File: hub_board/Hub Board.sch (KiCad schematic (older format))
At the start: 23 parts, among them J1 Conn_01x04, J2 Conn_01x04, J3 Conn_01x04, J4 Conn_01x04, P4 SERIAL, SW1 Switch_SPDT_x2, SW2 Switch_DPST, U0 10118194, U1 LM3671, U3 ESP-12E, U4 DIY-OLED-0.96, U5 SF303GJ26, U6 SN74LVC1T45 - MOSI, U7 SN74LVC1T45 - SCLK

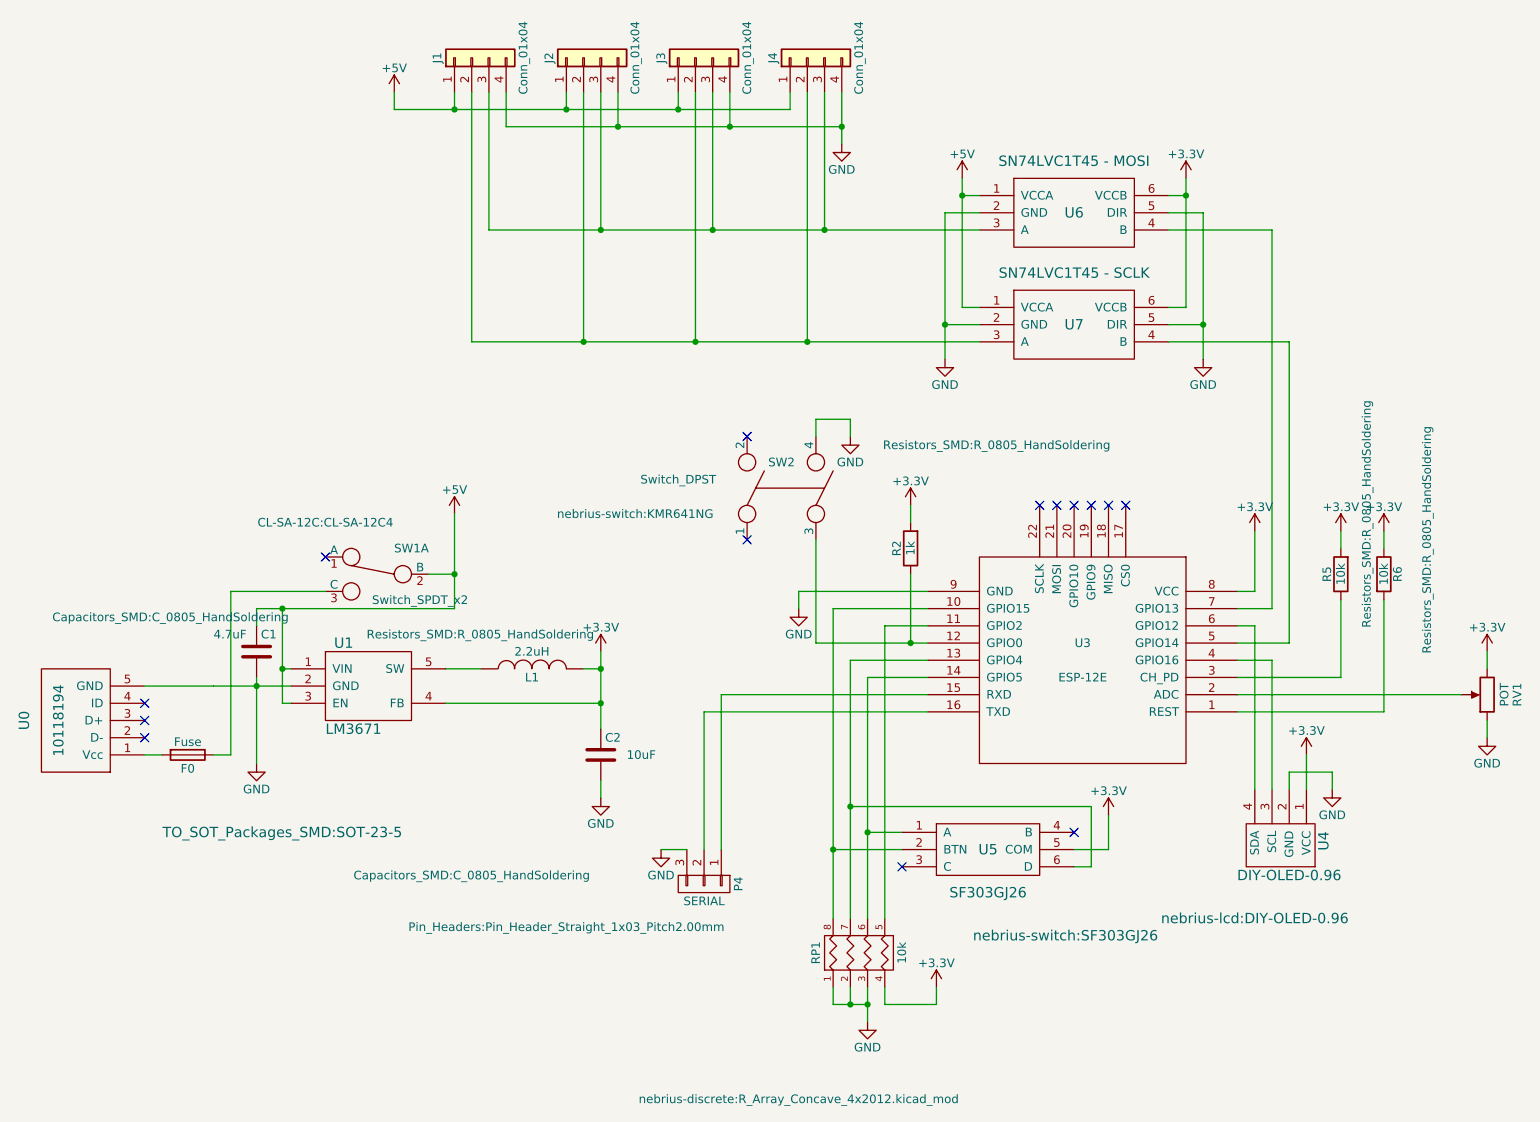
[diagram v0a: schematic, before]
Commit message: Forgot to add unsaved changes
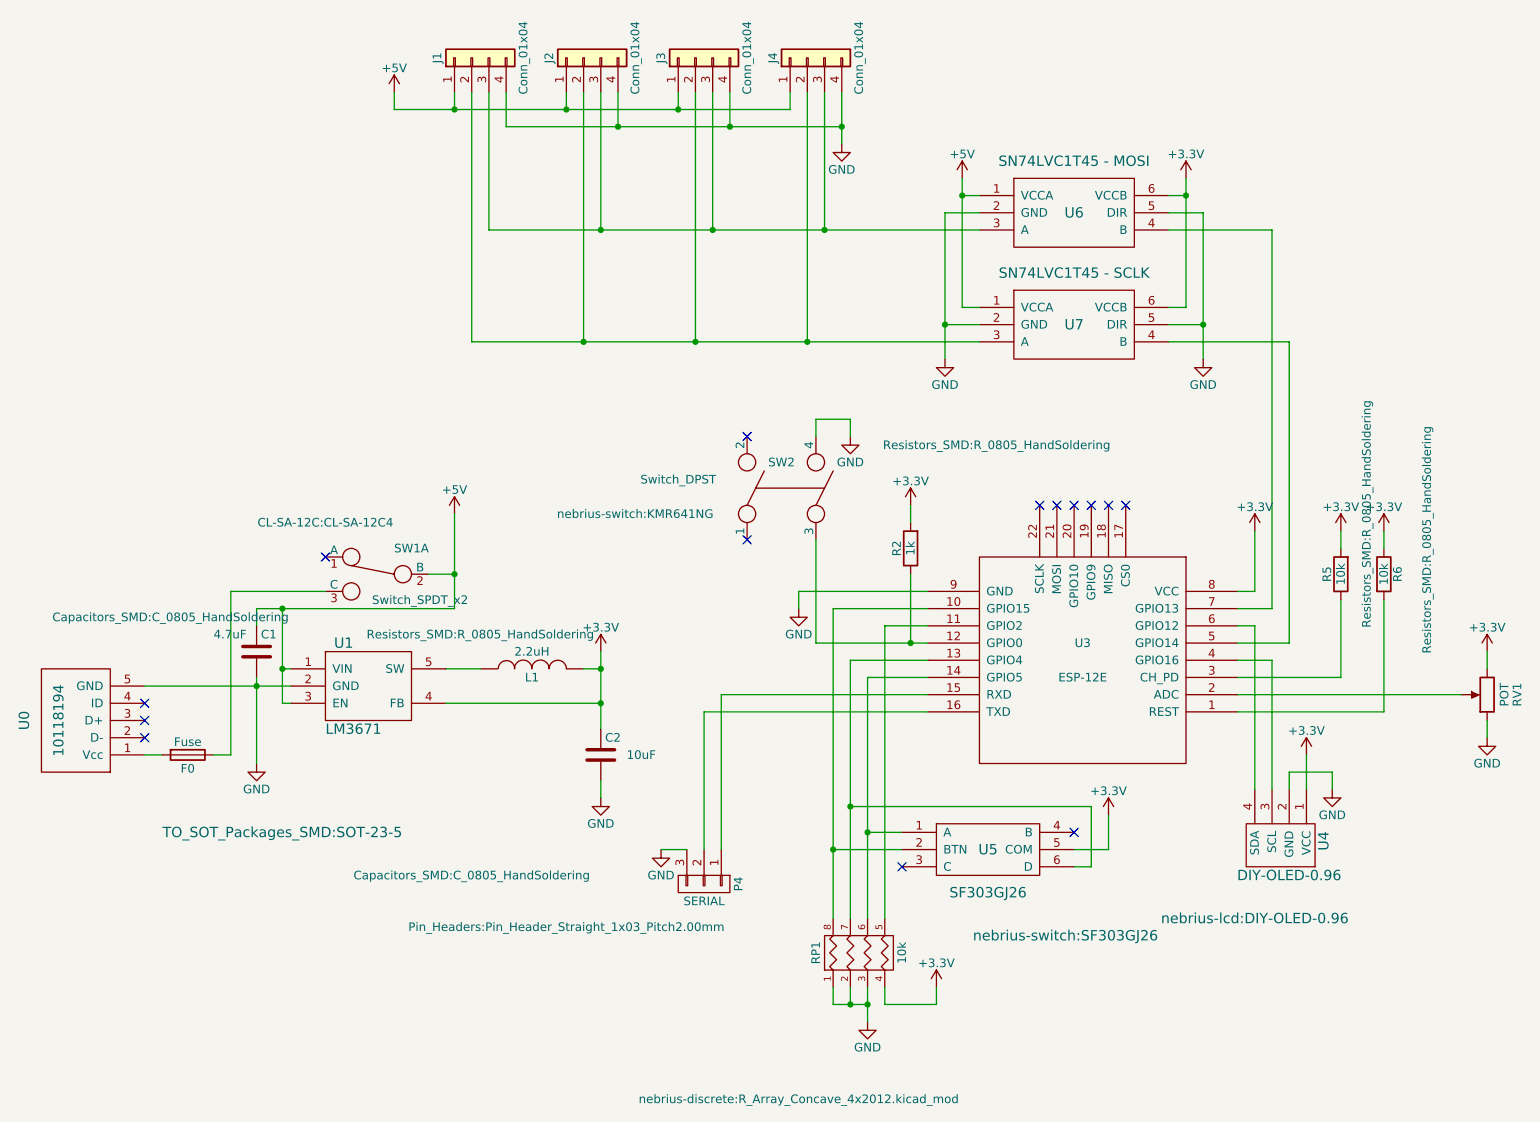
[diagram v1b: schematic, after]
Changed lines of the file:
@@
 Connection ~ 2000 4700
 Wire Wire Line
-	1850 4750 1850 4800
-Wire Wire Line
-	1850 4800 1850 5250
+	1850 4750 1850 5250
 Wire Wire Line
 	2950 4700 3150 4700
 Wire Wire Line
-	3000 4350 3000 4150
-Wire Wire Line
-	3000 4150 3000 3800
-Wire Wire Line
-	1850 4350 2000 4350
-Wire Wire Line
-	2000 4350 3000 4350
+	3000 4350 3000 3800
+Wire Wire Line
+	1850 4350 3000 4350
 Wire Wire Line
 	1850 4350 1850 4450
 Connection ~ 2000 4350
 Wire Wire Line
-	3850 4600 3850 4700
-Wire Wire Line
-	3850 4700 3850 4900
-Wire Wire Line
-	3850 4900 3850 5050
+	3850 4600 3850 5050
 Wire Wire Line
 	2950 4900 3850 4900
@@
 	4550 4850 4550 5750
 Wire Wire Line
-	5100 4550 5650 4550
-Wire Wire Line
-	5650 4550 5750 4550
+	5100 4550 5750 4550
 Wire Wire Line
 	5650 4150 5650 4550
@@
 	5300 3250 5300 3350
 Wire Wire Line
-	1600 4800 1200 4800
+	1200 4800 2050 4800
 Connection ~ 3000 4150
 Wire Wire Line
@@
 	3000 1450 3000 1350
 Wire Wire Line
-	2650 1450 3000 1450
-Wire Wire Line
-	3000 1450 3650 1450
-Wire Wire Line
-	3650 1450 4300 1450
-Wire Wire Line
-	4300 1450 4950 1450
+	2650 1450 4950 1450
 Wire Wire Line
 	2650 1450 2650 1350
@@
 Connection ~ 3650 1450
 Wire Wire Line
-	5250 1350 5250 1550
-Wire Wire Line
-	5250 1550 5250 1650
+	5250 1350 5250 1650
 Wire Wire Line
 	3950 1550 3950 1350
@@
 Connection ~ 3950 1550
 Wire Wire Line
-	5950 1850 5950 1950
-Wire Wire Line
-	5950 1950 5950 2600
+	5950 1850 5950 2600
 Wire Wire Line
 	5950 1950 6050 1950
@@
 Connection ~ 5950 1950
 Wire Wire Line
-	7250 1850 7250 1950
-Wire Wire Line
-	7250 1950 7250 2600
+	7250 1850 7250 2600
 Wire Wire Line
 	7250 1950 7150 1950
@@
 	7150 2050 7350 2050
 Wire Wire Line
-	7350 2050 7350 2700
-Wire Wire Line
-	7350 2700 7350 2900
+	7350 2050 7350 2900
 Wire Wire Line
 	7150 2700 7350 2700
@@
 	6050 2050 5850 2050
 Wire Wire Line
-	5850 2050 5850 2700
-Wire Wire Line
-	5850 2700 5850 2900
+	5850 2050 5850 2900
 Wire Wire Line
 	6050 2700 5850 2700
 Connection ~ 5850 2700
 Wire Wire Line
-	3200 2150 3850 2150
-Wire Wire Line
-	3850 2150 4500 2150
-Wire Wire Line
-	4500 2150 5150 2150
-Wire Wire Line
-	5150 2150 6050 2150
-Wire Wire Line
-	3100 2800 3750 2800
-Wire Wire Line
-	3750 2800 4400 2800
-Wire Wire Line
-	4400 2800 5050 2800
-Wire Wire Line
-	5050 2800 6050 2800
+	3200 2150 6050 2150
+Wire Wire Line
+	3100 2800 6050 2800
 Wire Wire Line
 	1200 5200 1300 5200
@@
 NoConn ~ 6400 3750
 Wire Wire Line
-	5200 4350 5200 5750
-Wire Wire Line
-	5200 5750 5200 6150
+	5200 4350 5200 6150
 $Comp
 L SF303GJ26 U5
@@
 $EndComp
 Wire Wire Line
-	5400 6550 5400 6650
-Wire Wire Line
-	5400 6650 5400 6750
+	5400 6550 5400 6750
 Wire Wire Line
 	5300 6550 5300 6650
@@
 	5750 4650 5300 4650
 Wire Wire Line
-	5300 4650 5300 5500
-Wire Wire Line
-	5300 5500 5300 6150
+	5300 4650 5300 6150
 Wire Wire Line
 	5750 4750 5400 4750
 Wire Wire Line
-	5400 4750 5400 5650
-Wire Wire Line
-	5400 5650 5400 6150
+	5400 4750 5400 6150
 Wire Wire Line
 	6600 5750 6800 5750
@@
 	7650 4450 7650 5400
 Wire Wire Line
-	5200 6650 5300 6650
-Wire Wire Line
-	5300 6650 5400 6650
+	5200 6650 5400 6650
 Wire Wire Line
 	5500 6550 5500 6650
@@
 	7550 4850 8850 4850
 Wire Wire Line
-	3300 1550 3950 1550
-Wire Wire Line
-	3950 1550 4600 1550
-Wire Wire Line
-	4600 1550 5250 1550
+	3300 1550 5250 1550
 $Comp
 L Conn_01x04 J3
@@
 Wire Wire Line
 	7150 2800 7850 2800
-Wire Wire Line
-	1600 4800 1850 4800
-Wire Wire Line
-	1850 4800 2050 4800
 Connection ~ 1850 4800
 Wire Wire Line
@@
 	2000 4900 2050 4900
 Wire Wire Line
-	2000 4350 2000 4700
-Wire Wire Line
-	2000 4700 2000 4900
+	2000 4350 2000 4900
 $EndSCHEMATC
